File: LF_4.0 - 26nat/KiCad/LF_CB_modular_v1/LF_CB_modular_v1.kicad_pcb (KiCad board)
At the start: 2 copper layers, 62 x 100 mm, 30 parts, among them J1 Conn_QTR16, J10 Conn_01x02, J11 Conn_01x10, J2 Conn_Arducam_MEGA_3mpx, J3 Conn_TB6612FNG_IC, J4 Conn_01x02, J5 Conn_01x05, J6 Conn_01x05, J8 Conn_01x01, J9 Conn_01x01, M1 Motor_DC, M2 Motor_DC, Q1 IRF4905, SW1 SW_SPDT, U1 Teensy4.1, U2 LM2940CT-5.0 _TO220, U3 TSR_1-2433

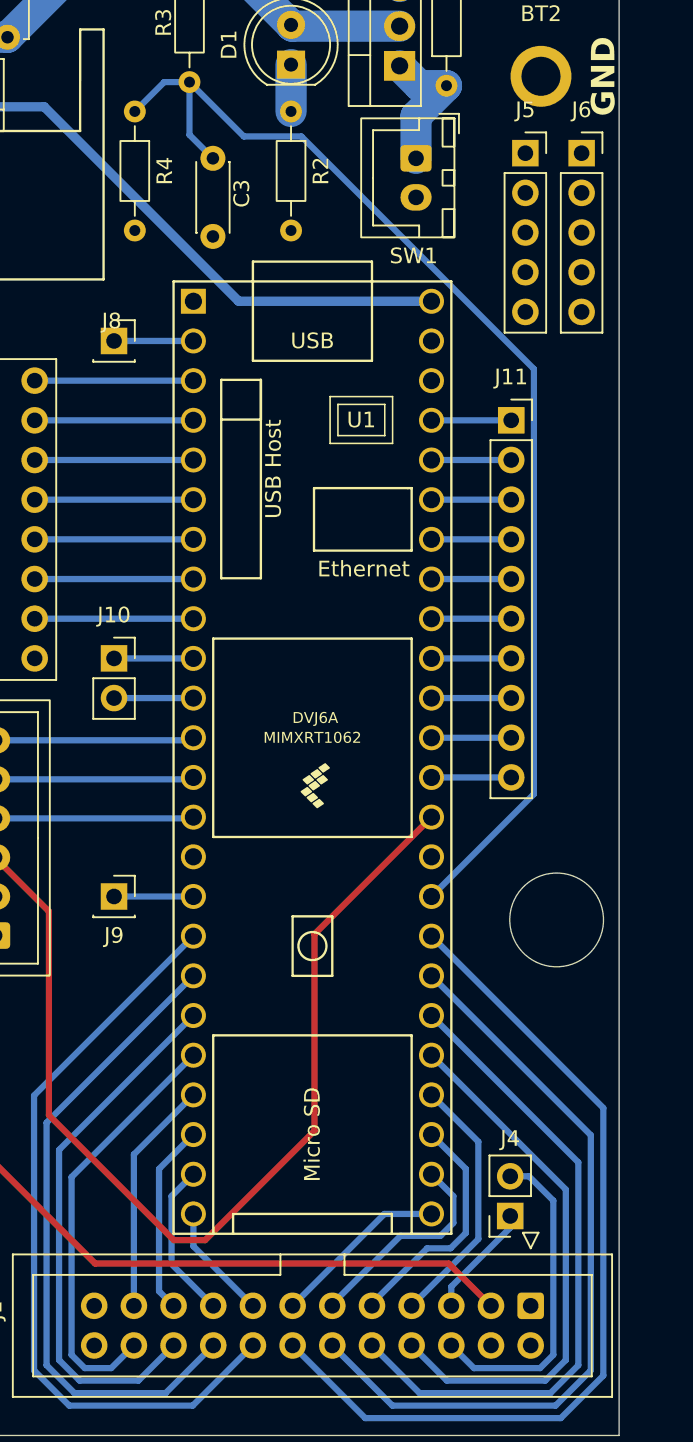
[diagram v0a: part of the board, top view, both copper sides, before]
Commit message: some last edits
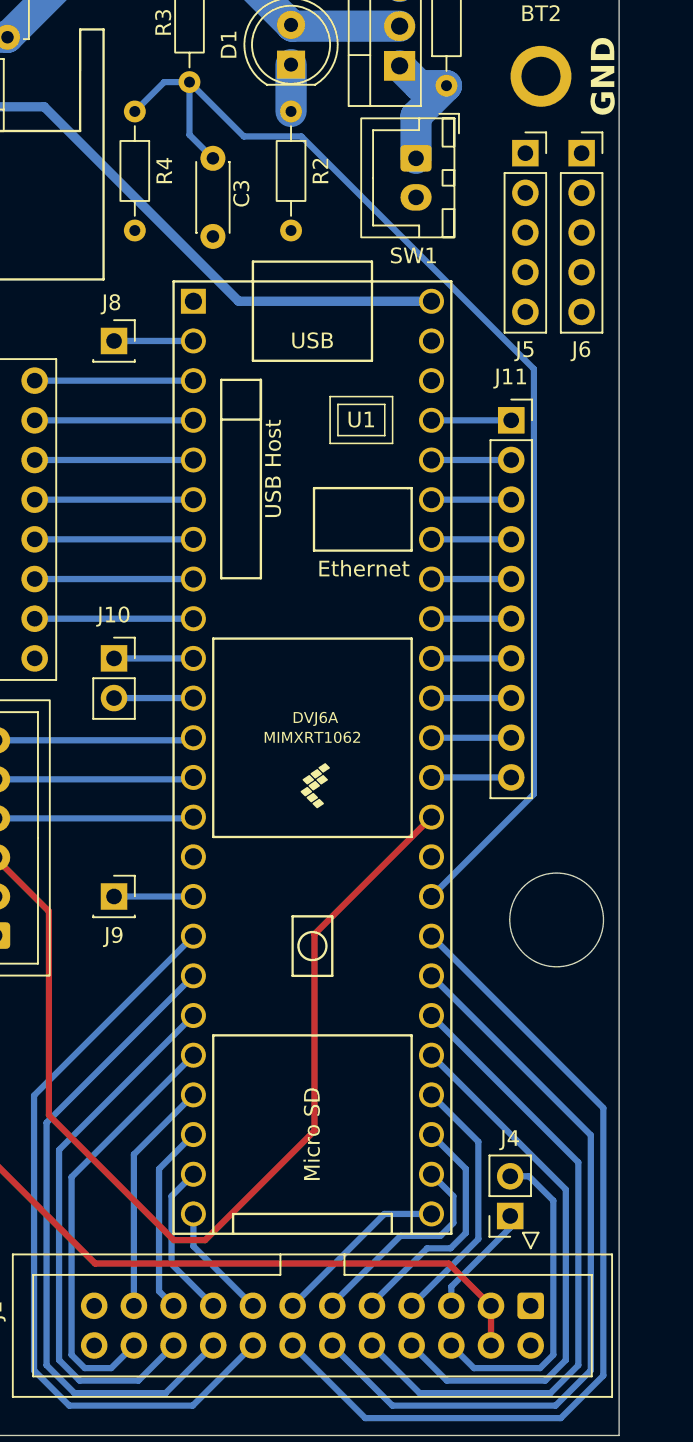
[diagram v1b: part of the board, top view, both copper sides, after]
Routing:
- net /3V3: track 92.0 -> 94.5 mm
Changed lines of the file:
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@@
 			)
 		)
+		(model "${KICAD9_3DMODEL_DIR}/Linefollower.3dshapes/Teensy 4.1 (With Headers).step"
+			(offset
+				(xyz 0 0 12)
+			)
+			(scale
+				(xyz 1 1 1)
+			)
+			(rotate
+				(xyz -0 -0 -0)
+			)
+		)
 	)
 	(footprint "Resistor_THT:R_Axial_DIN0204_L3.6mm_D1.6mm_P7.62mm_Horizontal"
@@
 		(tags "Through hole socket strip THT 1x05 2.54mm single row")
 		(property "Reference" "J5"
-			(at 0 -2.77 0)
+			(at 0 12.58 0)
 			(layer "F.SilkS")
 			(effects
@@
 		(tags "Through hole socket strip THT 1x05 2.54mm single row")
 		(property "Reference" "J6"
-			(at 0 -2.77 0)
+			(at 0 12.58 0)
 			(layer "F.SilkS")
 			(effects
@@
 		(model "${KICAD9_3DMODEL_DIR}/LED_THT.3dshapes/LED_D5.0mm.step"
 			(offset
-				(xyz 0 0 0)
+				(xyz 0 0 -3)
 			)
 			(scale
@@
 			)
 			(rotate
-				(xyz 0 0 0)
+				(xyz -0 -0 -0)
 			)
 		)
@@
 		(tags "Through hole socket strip THT 1x01 2.54mm single row")
 		(property "Reference" "J8"
-			(at -0.15 -1.27 0)
+			(at -0.15 -2.44 0)
 			(layer "F.SilkS")
 			(effects
@@
 	)
 	(segment
+		(start 89.8 132.7)
+		(end 89.8 135.24)
+		(width 0.4)
+		(layer "F.Cu")
+		(net 15)
+	)
+	(segment
